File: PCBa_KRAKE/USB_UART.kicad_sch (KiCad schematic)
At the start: 19 parts, among them J501 USB_B_Micro_Local, Q998 MMBT2222ALT1G, Q999 MMBT2222ALT1G, U501 CH340T

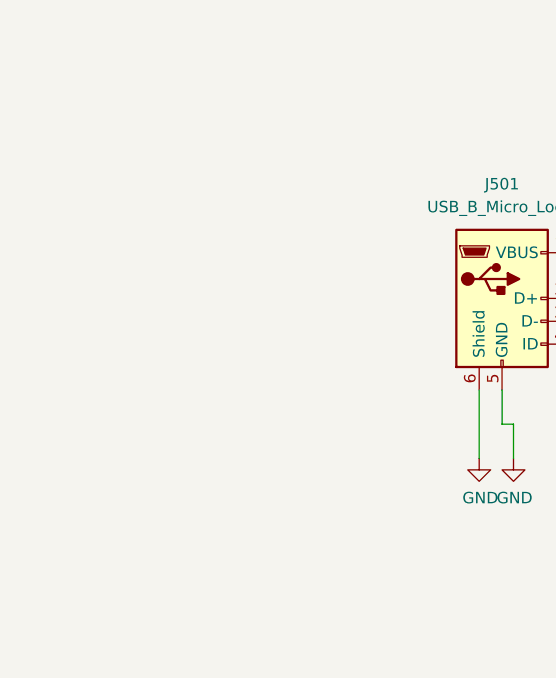
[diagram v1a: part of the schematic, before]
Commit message: Added 5V to 3v3 level shifters to SPI bus.Added but not wired a USBc connector.
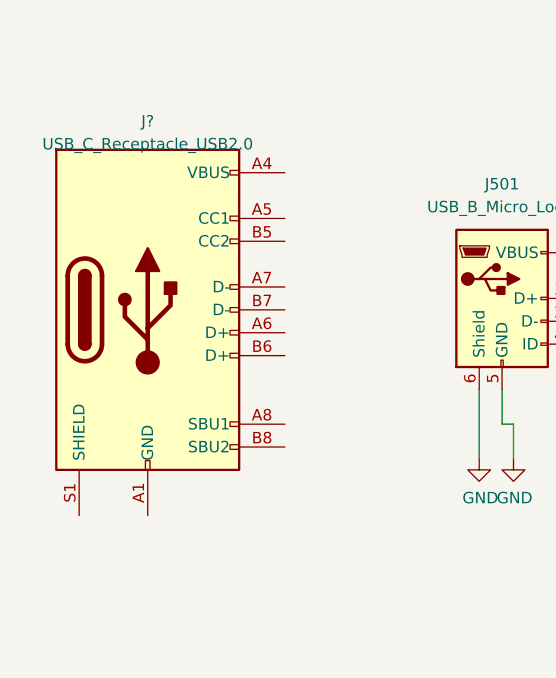
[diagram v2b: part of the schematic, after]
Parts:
- added J?: USB_C_Receptacle_USB2.0, symbol Connector:USB_C_Receptacle_USB2.0
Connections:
- new net: J?.A1 (GND), J?.A12 (GND), J?.B1 (GND), J?.B12 (GND)
- new net: J?.A4 (VBUS), J?.A9 (VBUS), J?.B4 (VBUS), J?.B9 (VBUS)
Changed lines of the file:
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@@
+    )
+  )
+  (symbol (lib_id "Connector:USB_C_Receptacle_USB2.0") (at 53.34 96.52 0) (unit 1)
+    (in_bom yes) (on_board yes) (dnp no) (fields_autoplaced)
+    (property "Reference" "J?" (at 53.34 75.565 0)
+      (effects (font (size 1.27 1.27)))
+    )
+    (property "Value" "USB_C_Receptacle_USB2.0" (at 53.34 78.105 0)
+      (effects (font (size 1.27 1.27)))
+    )
+    (property "Footprint" "" (at 57.15 96.52 0)
+      (effects (font (size 1.27 1.27)) hide)
+    )
+    (property "Datasheet" "https://www.usb.org/sites/default/files/documents/usb_type-c.zip" (at 57.15 96.52 0)
+      (effects (font (size 1.27 1.27)) hide)
+    )
+    (pin "A1")
+    (pin "A12")
+    (pin "A4")
+    (pin "A5")
+    (pin "A6")
+    (pin "A7")
+    (pin "A8")
+    (pin "A9")
+    (pin "B1")
+    (pin "B12")
+    (pin "B4")
+    (pin "B5")
+    (pin "B6")
+    (pin "B7")
+    (pin "B8")
+    (pin "B9")
+    (pin "S1")
+    (instances
+      (project "PCBa_KRAKE"
+        (path "/412a327d-1ee3-473e-bc00-1545004b7edf"
+          (reference "J?") (unit 1)
+        )
+        (path "/412a327d-1ee3-473e-bc00-1545004b7edf/00000000-0000-0000-0000-000062bc4e7e"
+          (reference "J?") (unit 1)
+        )
+      )
     )
   )

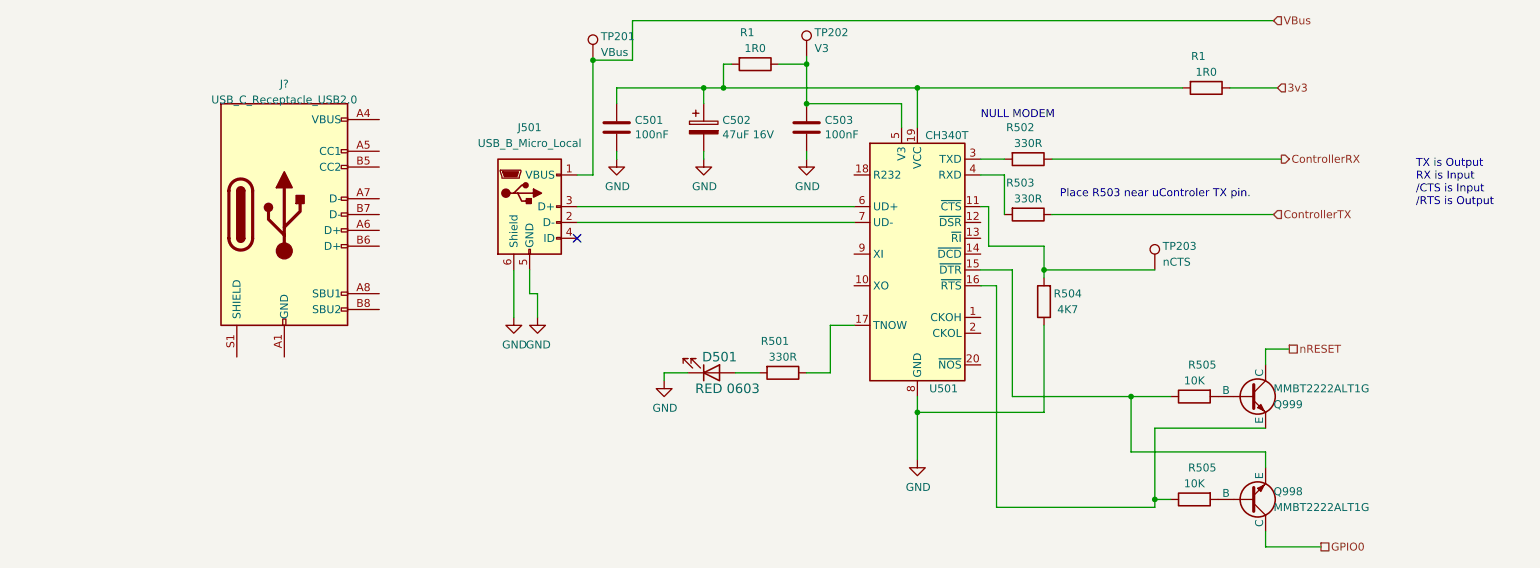
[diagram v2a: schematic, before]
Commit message: Editted USB C schematic symbol. Replaced the USB B with the USB C.
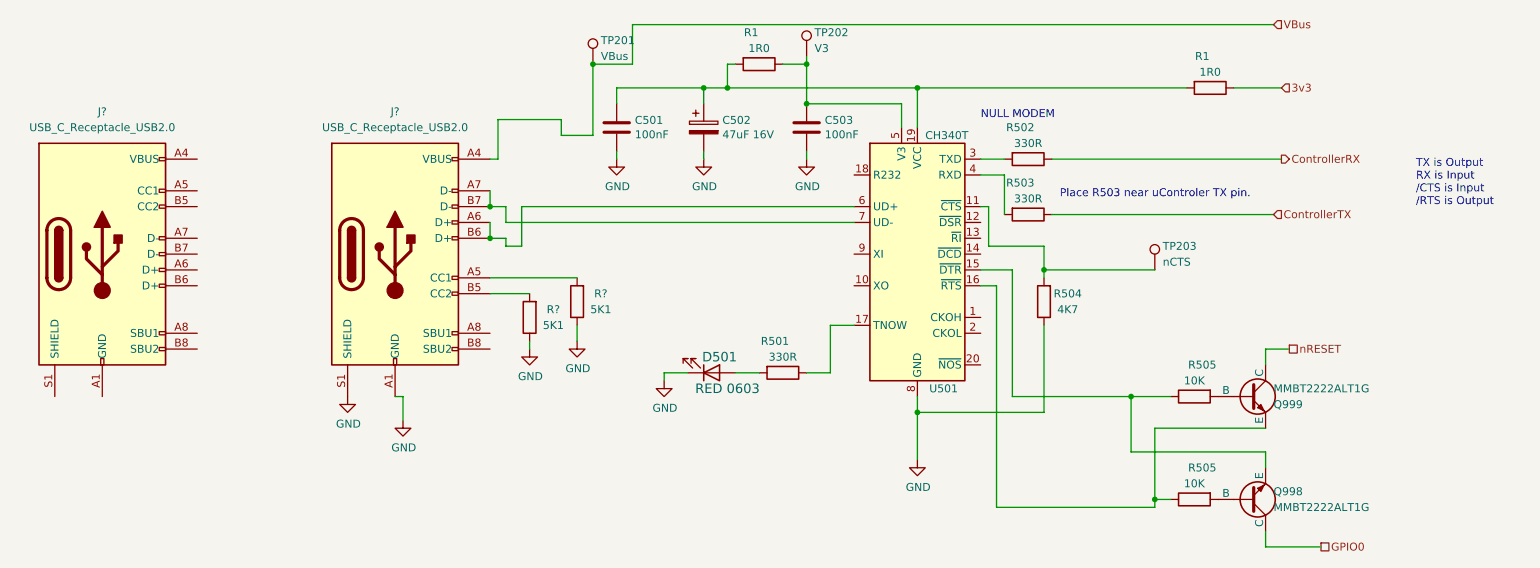
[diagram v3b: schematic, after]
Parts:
- removed J501: USB_B_Micro_Local, GeneralPurposeAlarmDevicePCB:USB_Micro-B_Amphenol_10118194_Horizontal, symbol GPAD_SCH_LIB:USB_B_Micro_Local
- removed J?: USB_C_Receptacle_USB2.0, symbol Connector:USB_C_Receptacle_USB2.0
- added J?: USB_C_Receptacle_USB2.0, symbol Connector:USB_C_Receptacle_USB2.0
- added J?: USB_C_Receptacle_USB2.0, symbol GPAD_SCH_LIB:USB_C_Receptacle_USB2.0_GPAD
- added R? (x2): 5K1, Resistor_SMD:R_0603_1608Metric_Pad0.98x0.95mm_HandSolder, symbol Device:R
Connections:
- net GND: now also J?.A1 (GND), J?.A12 (GND), J?.B1 (GND), J?.B12 (GND), J?.S1 (SHIELD), R?.1, R?.1
- net VBus: now also J?.A4 (VBUS), J?.A9 (VBUS), J?.B4 (VBUS), J?.B9 (VBUS)
- net at U501.7 (UD-): now also J?.A7 (D-), J?.B7 (D-)
- net at U501.6 (UD+): now also J?.A6 (D+), J?.B6 (D+)
- new net: J?.A1 (GND), J?.A12 (GND), J?.B1 (GND), J?.B12 (GND)
- new net: J?.A4 (VBUS), J?.A9 (VBUS), J?.B4 (VBUS), J?.B9 (VBUS)
- new net: J?.A5 (CC1), R?.2
- new net: J?.B5 (CC2), R?.2
- no-connect marks 1 -> 0
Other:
- moved on the sheet: R1, TP201
